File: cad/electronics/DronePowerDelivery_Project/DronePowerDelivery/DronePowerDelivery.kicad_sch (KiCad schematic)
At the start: 0 parts

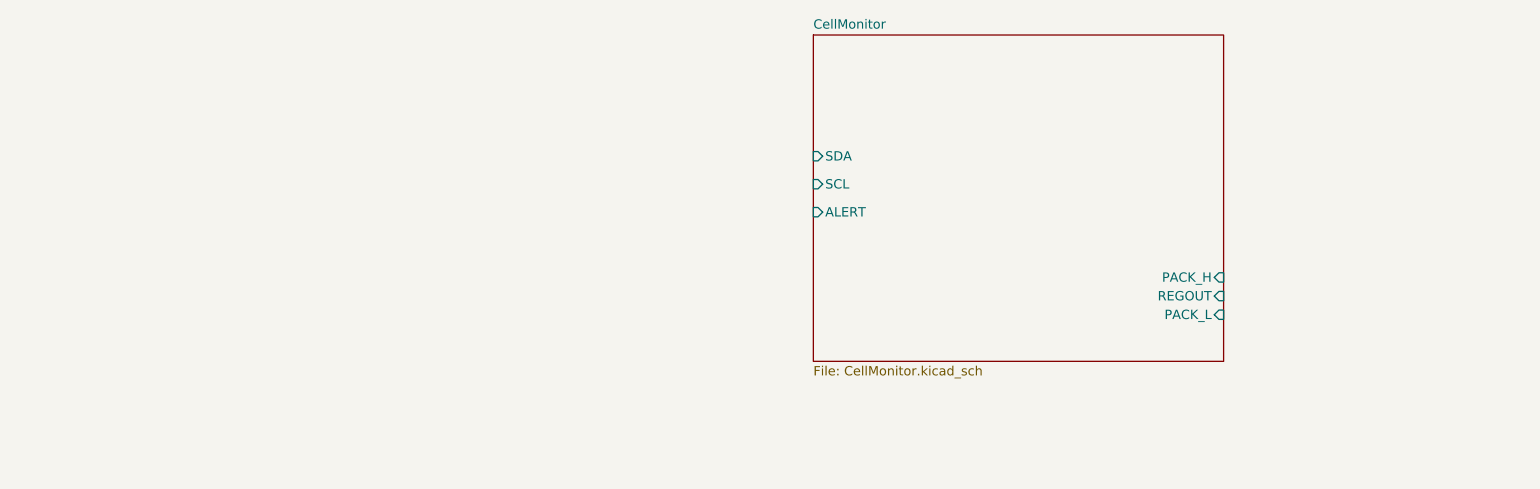
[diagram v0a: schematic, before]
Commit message: Finialized Component Sizing
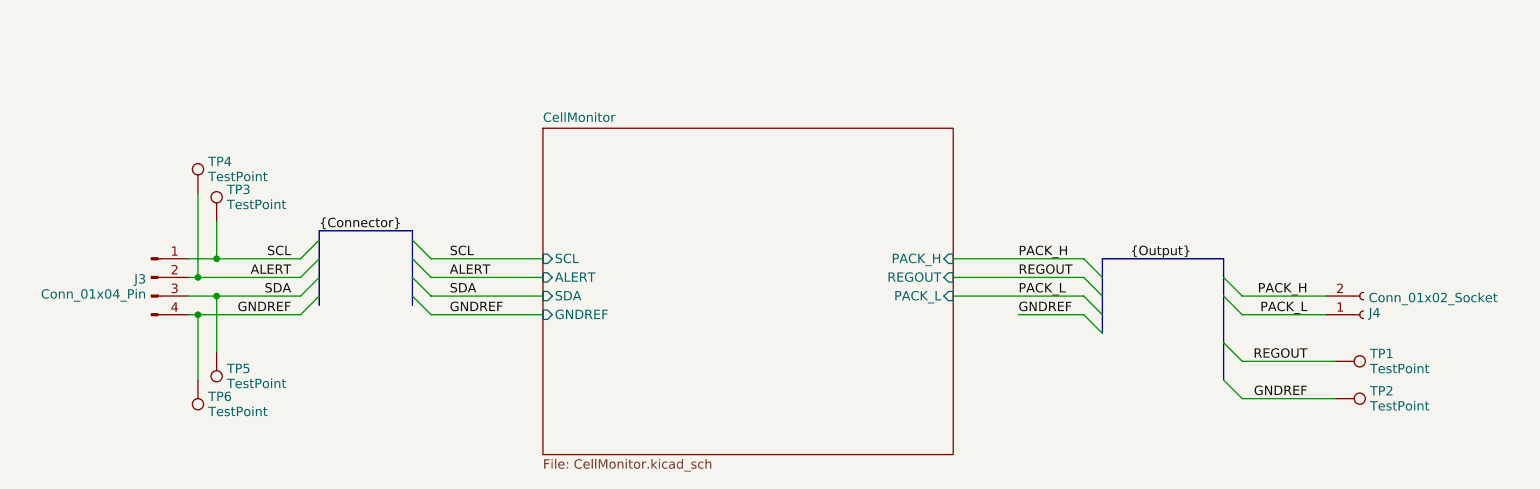
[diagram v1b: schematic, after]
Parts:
- added J3: Conn_01x04_Pin, Connector_JST:JST_PH_B4B-PH-K_1x04_P2.00mm_Vertical, symbol Connector:Conn_01x04_Pin
- added J4: Conn_01x02_Socket, Connector_AMASS:AMASS_XT60-M_1x02_P7.20mm_Vertical, symbol Connector:Conn_01x02_Socket
- added TP1, TP2, TP3, TP4, TP5, TP6: TestPoint, TestPoint:TestPoint_Pad_3.0x3.0mm, symbol Connector:TestPoint
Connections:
- new net ALERT: J3.2 (Pin_2), TP4.1
- new net GNDREF: J3.4 (Pin_4), TP2.1, TP6.1
- new net PACK_H: J4.2 (Pin_2)
- new net PACK_L: J4.1 (Pin_1)
- new net REGOUT: TP1.1
- new net SCL: J3.1 (Pin_1), TP3.1
- new net SDA: J3.3 (Pin_3), TP5.1
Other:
- sheet CellMonitor ports: added GNDREF; removed none

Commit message: Rev.1 of PCB laid out
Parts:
- TP1, TP2, TP3, TP4, TP5, TP6: footprint TestPoint:TestPoint_Pad_3.0x3.0mm -> TestPoint:TestPoint_Pad_2.0x2.0mm
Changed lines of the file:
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@@
 (kicad_sch (version 20230121) (generator eeschema)
   (paper "A4")
+  (bus_alias "Connector" (members "SCL" "ALERT" "SDA" "GNDREF"))
   (bus_alias "Output" (members "PACK_H" "PACK_L" "REGOUT" "GNDREF"))
-  (bus_alias "Connector" (members "SCL" "ALERT" "SDA" "GNDREF"))
   (junction (at 72.39 86.36) (diameter 0) (color 0 0 0 0)
   )
@@
     (effects (font (size 1.27 1.27)) (justify right bottom))
   )
+  (netclass_flag "" (length 2.54) (shape round) (at 222.25 91.44 0) (fields_autoplaced)
+    (effects (font (size 1.27 1.27)) (justify left bottom))
+    (property "Netclass" "Power" (at 222.9485 88.9 0)
+      (effects (font (size 1.27 1.27) italic) (justify left))
+    )
+  )
+  (netclass_flag "" (length 2.54) (shape round) (at 222.25 93.98 180) (fields_autoplaced)
+    (effects (font (size 1.27 1.27)) (justify right bottom))
+    (property "Netclass" "Power" (at 222.9485 96.52 0)
+      (effects (font (size 1.27 1.27) italic) (justify left))
+    )
+  )
   (symbol (lib_id "Connector:TestPoint") (at 69.85 77.47 0) (unit 1)
     (in_bom yes) (on_board yes) (dnp no) (fields_autoplaced)
@@
       (effects (font (size 1.27 1.27)) (justify left))
     )
-    (property "Footprint" "TestPoint:TestPoint_Pad_3.0x3.0mm" (at 74.93 77.47 0)
+    (property "Footprint" "TestPoint:TestPoint_Pad_2.0x2.0mm" (at 74.93 77.47 0)
       (effects (font (size 1.27 1.27)) hide)
     )
@@
       (effects (font (size 1.27 1.27)) (justify right))
     )
-    (property "Footprint" "TestPoint:TestPoint_Pad_3.0x3.0mm" (at 67.31 99.06 0)
+    (property "Footprint" "TestPoint:TestPoint_Pad_2.0x2.0mm" (at 67.31 99.06 0)
       (effects (font (size 1.27 1.27)) hide)
     )
@@
       (effects (font (size 1.27 1.27)) (justify left))
     )
-    (property "Footprint" "TestPoint:TestPoint_Pad_3.0x3.0mm" (at 224.79 110.49 0)
+    (property "Footprint" "TestPoint:TestPoint_Pad_2.0x2.0mm" (at 224.79 110.49 0)
       (effects (font (size 1.27 1.27)) hide)
     )
@@
       (effects (font (size 1.27 1.27)) (justify right))
     )
-    (property "Footprint" "TestPoint:TestPoint_Pad_3.0x3.0mm" (at 64.77 102.87 0)
+    (property "Footprint" "TestPoint:TestPoint_Pad_2.0x2.0mm" (at 64.77 102.87 0)
       (effects (font (size 1.27 1.27)) hide)
     )
@@
       (effects (font (size 1.27 1.27)) (justify left))
     )
-    (property "Footprint" "TestPoint:TestPoint_Pad_3.0x3.0mm" (at 224.79 105.41 0)
+    (property "Footprint" "TestPoint:TestPoint_Pad_2.0x2.0mm" (at 224.79 105.41 0)
       (effects (font (size 1.27 1.27)) hide)
     )
@@
       (effects (font (size 1.27 1.27)) (justify left))
     )
-    (property "Footprint" "TestPoint:TestPoint_Pad_3.0x3.0mm" (at 77.47 81.28 0)
-      (effects (font (size 1.27 1.27)) hide)
-    )
+    (property "Footprint" "TestPoint:TestPoint_Pad_2.0x2.0mm" (at 77.47 81.28 0)
+      (effects (font (size 1.27 1.27)) hide)
+    )
